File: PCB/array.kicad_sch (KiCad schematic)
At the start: 9 parts

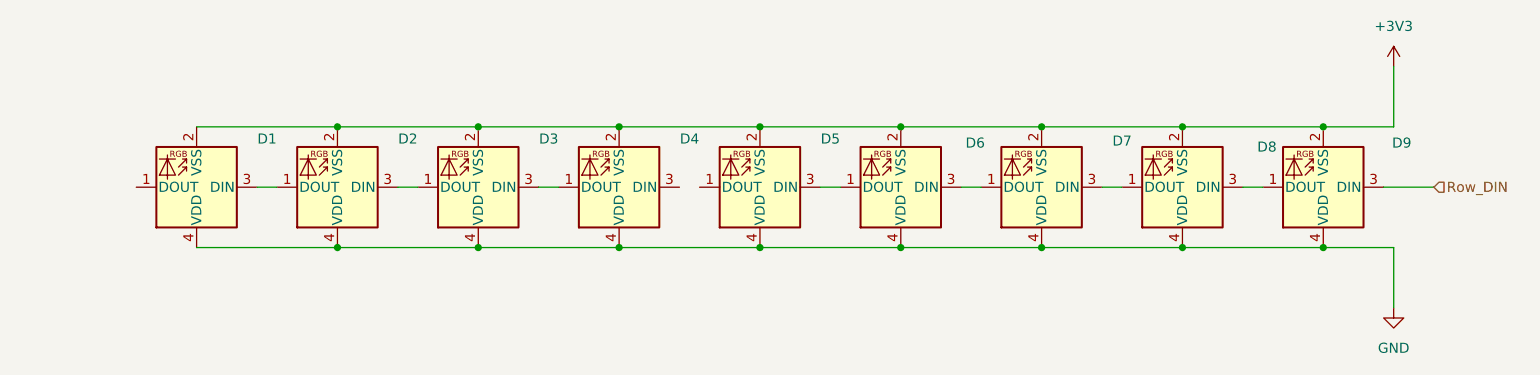
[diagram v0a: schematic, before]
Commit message: Made first PCB
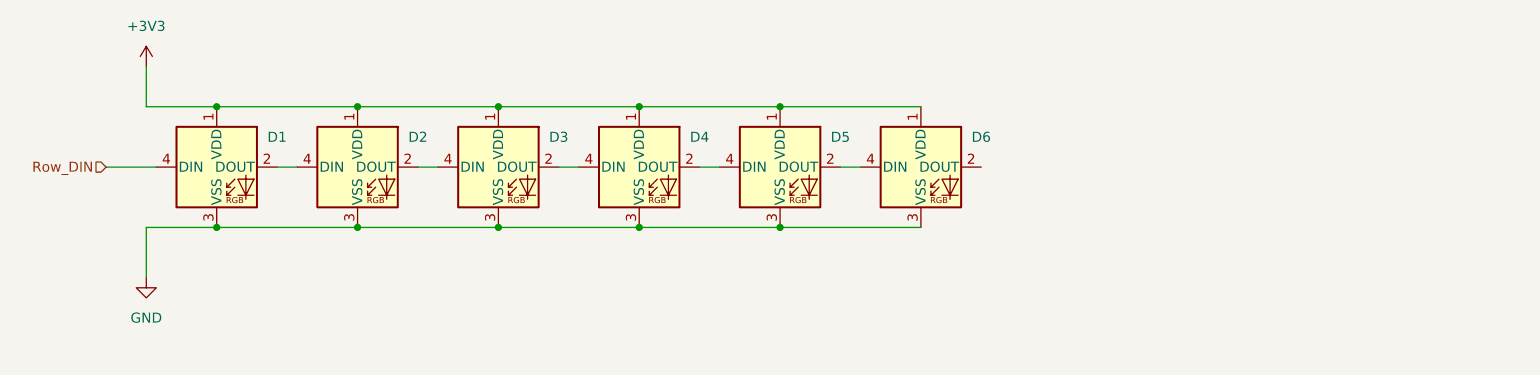
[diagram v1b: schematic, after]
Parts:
- removed D1, D2, D3, D4, D5, D6, D7, D8, D9: WS2812B-2020, LED_SMD:LED_WS2812B-2020_PLCC4_2.0x2.0mm, symbol LED:WS2812B-2020
- added D1, D2, D3, D4, D5, D6: WS2812B, LED_SMD:LED_WS2812B_PLCC4_5.0x5.0mm_P3.2mm, symbol LED:WS2812B
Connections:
- net +3V3: now also D1.1 (VDD), D2.1 (VDD), D3.1 (VDD), D4.1 (VDD), D5.1 (VDD), D6.1 (VDD)
- net GND: now also D1.3 (VSS), D2.3 (VSS), D3.3 (VSS), D4.3 (VSS), D5.3 (VSS), D6.3 (VSS)
- net Row_DIN: now also D1.4 (DIN)
- new net: D2.2 (DOUT), D3.4 (DIN)
- new net: D1.2 (DOUT), D2.4 (DIN)
- new net: D3.2 (DOUT), D4.4 (DIN)
- new net: D5.2 (DOUT), D6.4 (DIN)
- new net: D4.2 (DOUT), D5.4 (DIN)

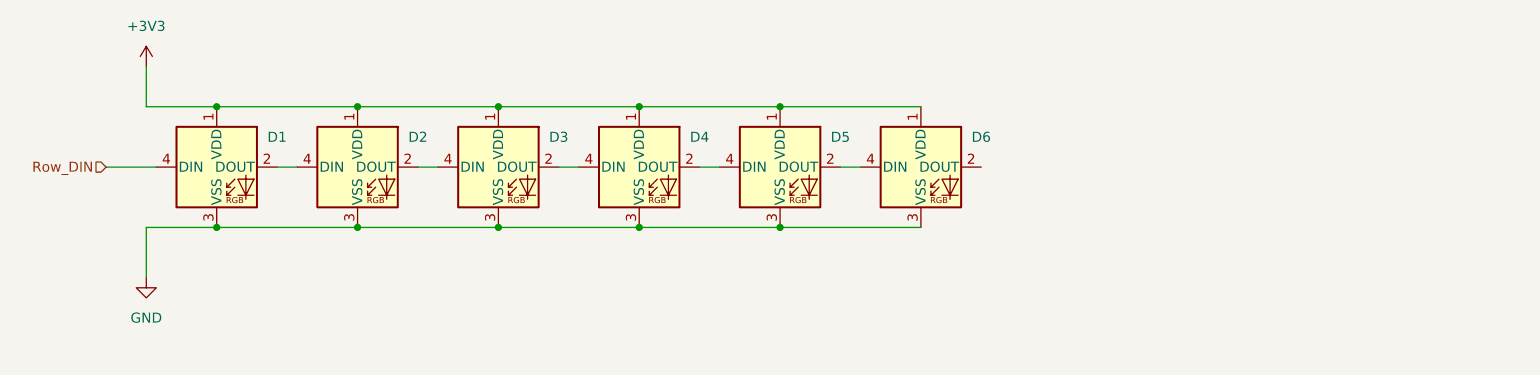
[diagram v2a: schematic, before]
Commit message: Made smol :) Anyway, this is just WIP, still working on it
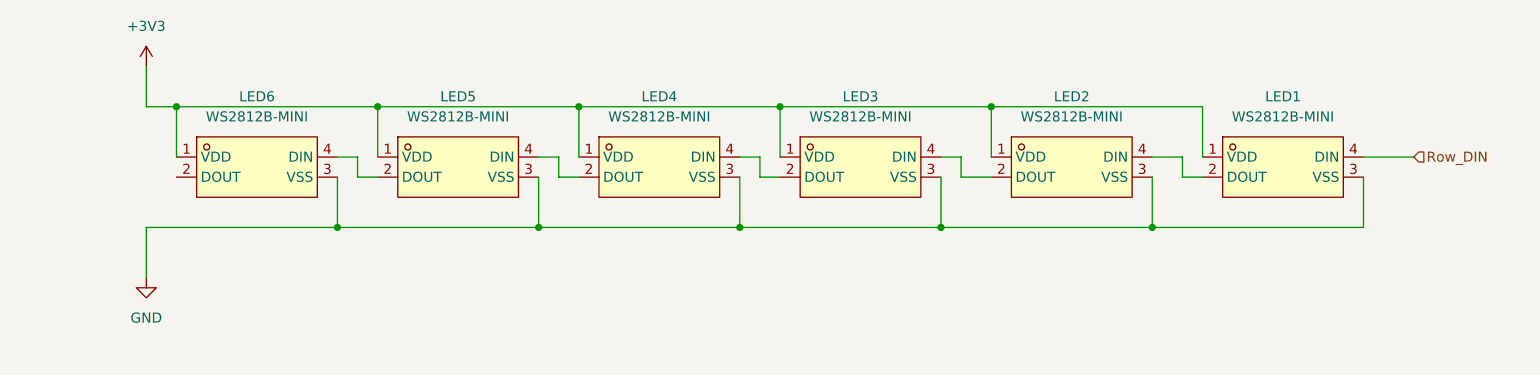
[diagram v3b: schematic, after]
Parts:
- removed D1, D2, D3, D4, D5, D6: WS2812B, LED_SMD:LED_WS2812B_PLCC4_5.0x5.0mm_P3.2mm, symbol LED:WS2812B
- added LED1, LED2, LED3, LED4, LED5, LED6: WS2812B-MINI, sponka:LED-SMD_4P-L3.5-W3.5-TL_WS2812B, symbol sponka:WS2812B-MINI
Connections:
- net +3V3: now also LED1.1 (VDD), LED2.1 (VDD), LED3.1 (VDD), LED4.1 (VDD), LED5.1 (VDD), LED6.1 (VDD)
- net GND: now also LED1.3 (VSS), LED2.3 (VSS), LED3.3 (VSS), LED4.3 (VSS), LED5.3 (VSS), LED6.3 (VSS)
- net Row_DIN: now also LED1.4 (DIN)
- new net: LED2.2 (DOUT), LED3.4 (DIN)
- new net: LED1.2 (DOUT), LED2.4 (DIN)
- new net: LED5.2 (DOUT), LED6.4 (DIN)
- new net: LED4.2 (DOUT), LED5.4 (DIN)
- new net: LED3.2 (DOUT), LED4.4 (DIN)
